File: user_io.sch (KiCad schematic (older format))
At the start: 20 parts

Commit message: Make updates per suggestions
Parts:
- removed J?: Conn_01x04, symbol Connector_Generic:Conn_01x04
- removed R? (x2): 0, symbol Device:R_Small
- removed SW?: SW_DPDT_x2, symbol Switch:SW_DPDT_x2
- removed SW?: SW_Push, symbol Switch:SW_Push
- added C11, C13: 20p, symbol Device:C_Small
- added C18, C19, C7, C9: 100n, symbol Device:C_Small
- added HSE1: 8MHz, symbol Device:Crystal_GND23_Small
- added J4: Conn_01x06_Male, symbol Connector:Conn_01x06_Male
- added J5: Conn_01x05_Male, symbol Connector:Conn_01x05_Male
- added J6, J8: Conn_01x04_Male, symbol Connector:Conn_01x04_Male
- added R12, R14, R15, R17, R18, R20, R21, R22: 10k, symbol Device:R_Small
- added R16: 390, symbol Device:R_Small
- added R19: 0, symbol Device:R_Small
- added SW1, SW2, SW3: SW_Push_Dual, symbol Switch:SW_Push_Dual
- gave numbers to parts that had none: 15
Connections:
- net labels added: OSC_IN, OSC_OUT, SPI_INT, SUBS_P_INT
- net labels removed: RA8875_3V_Out, RA8875_GND, RA8875_LITE, RA8875_VIN, RA8875_XM, RA8875_XP, RA8875_YM, RA8875_YP, SCREEN_INT, SCREEN_MISO, SCREEN_MOSI, SCREEN_NRST, SCREEN_NSS, SCREEN_SCK, SCREEN_WAIT
- wire segments 101 -> 182
- no-connect marks 47 -> 44
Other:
- note added: "External Oscillator"
- note added: "Serial Communication Header Pins\n"
- note added: "User IO to DAC SPI"
- note added: "User Pushbutton\n"
- note removed: "Known No-Connects"
- note removed: "Power/Gnd"
- note removed: "Signals"
- note removed: "USART Debug Connection"
- note removed: "User IO to DAC Subsystem Communication"
- moved on the sheet: C10, C12, C14, C15, C16, C17, C8, J3, J7, R11, R13, R23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

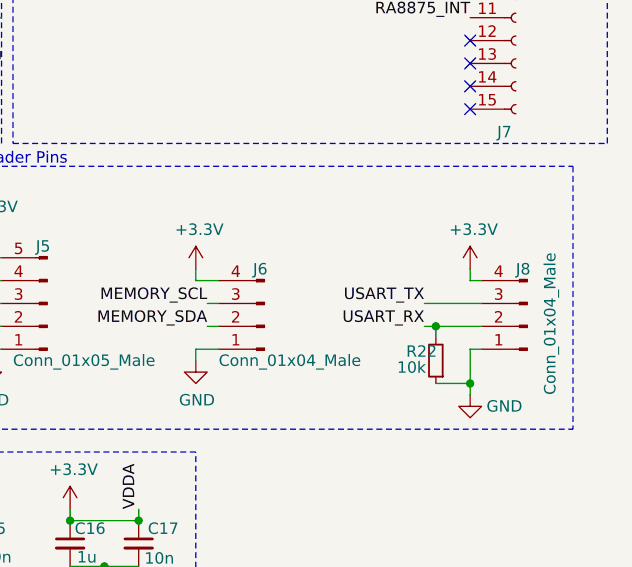
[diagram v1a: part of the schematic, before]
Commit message: Make most changes for final design
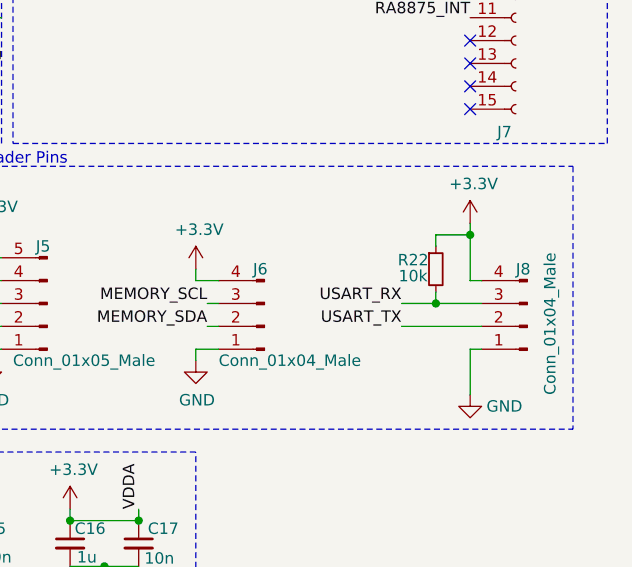
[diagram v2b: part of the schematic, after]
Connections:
- net +3V3: now also R22.1
- net GND: no longer R22.1
- net USART_RX: now also J8.3 (Pin_3); no longer J8.2 (Pin_2)
- net USART_TX: now also J8.2 (Pin_2); no longer J8.3 (Pin_3)
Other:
- moved on the sheet: R22
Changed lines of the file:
@@
 L power:+3.3V #PWR053
 U 1 1 6055EB95
-P 9900 4600
-F 0 "#PWR053" H 9900 4450 50  0001 C CNN
-F 1 "+3.3V" H 9915 4773 50  0000 C CNN
-F 2 "" H 9900 4600 50  0001 C CNN
-F 3 "" H 9900 4600 50  0001 C CNN
-	1    9900 4600
+P 9900 4400
+F 0 "#PWR053" H 9900 4250 50  0001 C CNN
+F 1 "+3.3V" H 9915 4573 50  0000 C CNN
+F 2 "" H 9900 4400 50  0001 C CNN
+F 3 "" H 9900 4400 50  0001 C CNN
+	1    9900 4400
 	1    0    0    -1
 $EndComp
@@
 	9900 4950 9950 4950
 Wire Wire Line
-	9900 4600 9900 4650
-Wire Wire Line
 	9900 4650 9950 4650
-Text Label 9700 4850 2    50   ~ 0
+Text Label 9600 4750 2    50   ~ 0
 USART_RX
-Text Label 9700 4750 2    50   ~ 0
+Text Label 9600 4850 2    50   ~ 0
 USART_TX
 Wire Notes Line
@@
 L Device:R_Small R22
 U 1 1 60A388CB
-P 9750 5000
-F 0 "R22" H 9880 4960 50  0000 R CNN
-F 1 "10k" H 9920 5030 50  0000 R CNN
-F 2 "" H 9750 5000 50  0001 C CNN
-F 3 "~" H 9750 5000 50  0001 C CNN
-	1    9750 5000
-	-1   0    0    1
-$EndComp
-Wire Wire Line
-	9750 5100 9900 5100
-Wire Wire Line
-	9900 5100 9900 5150
-Wire Wire Line
-	9750 4900 9750 4850
-Wire Wire Line
-	9750 4850 9950 4850
-Wire Wire Line
-	9700 4850 9750 4850
-Connection ~ 9750 4850
-Wire Wire Line
-	9900 4950 9900 5100
-Connection ~ 9900 5100
-Wire Wire Line
-	9700 4750 9950 4750
+P 9750 4600
+F 0 "R22" H 9718 4640 50  0000 R CNN
+F 1 "10k" H 9714 4570 50  0000 R CNN
+F 2 "" H 9750 4600 50  0001 C CNN
+F 3 "~" H 9750 4600 50  0001 C CNN
+	1    9750 4600
+	1    0    0    -1
+$EndComp
 Wire Notes Line
 	10350 4150 10350 5300
@@
 Text Notes 5400 700  0    50   ~ 0
 User Pushbutton\n
+Wire Wire Line
+	9900 4950 9900 5150
+Wire Wire Line
+	9600 4750 9750 4750
+Wire Wire Line
+	9600 4850 9950 4850
+Wire Wire Line
+	9750 4700 9750 4750
+Connection ~ 9750 4750
+Wire Wire Line
+	9750 4750 9950 4750
+Wire Wire Line
+	9750 4500 9750 4450
+Wire Wire Line
+	9750 4450 9900 4450
+Wire Wire Line
+	9900 4450 9900 4400
+Wire Wire Line
+	9900 4450 9900 4650
+Connection ~ 9900 4450
 $EndSCHEMATC
